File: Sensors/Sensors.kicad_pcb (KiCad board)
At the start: 4 copper layers, 17.6 x 37 mm, 11 parts, among them J1 Conn_01x05, J2 Conn_01x04, J3 Conn_01x02, U1 LIS2DE12, U2 MS5607-02BA

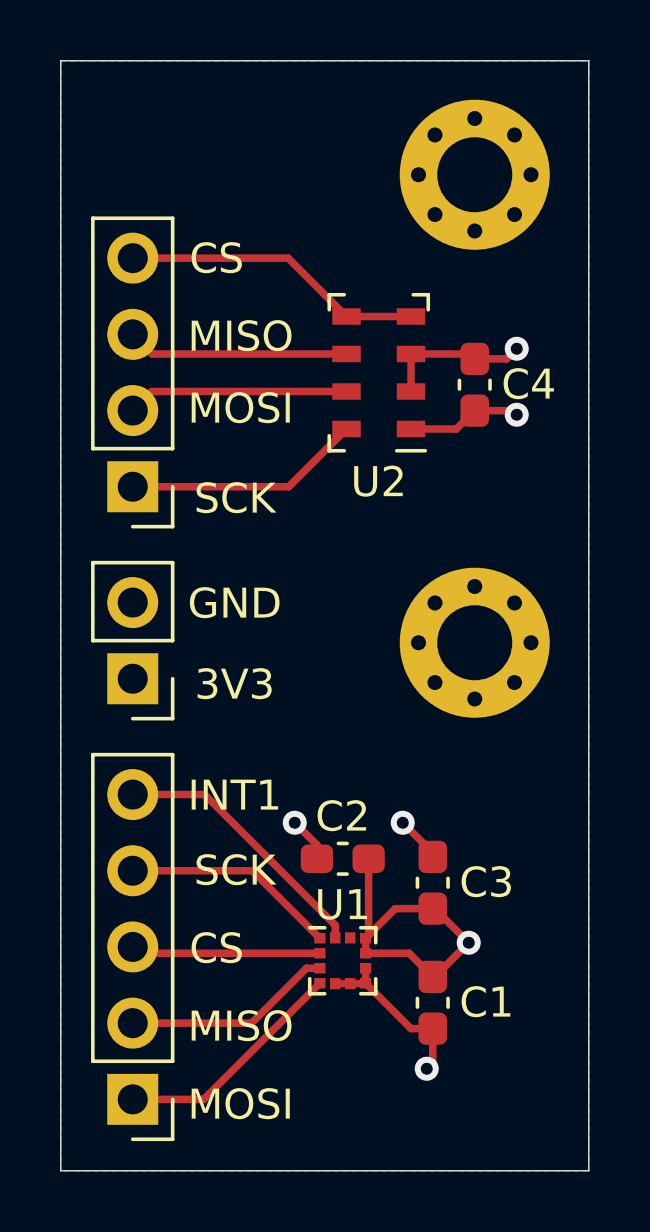
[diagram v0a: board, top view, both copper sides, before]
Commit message: Add files via upload
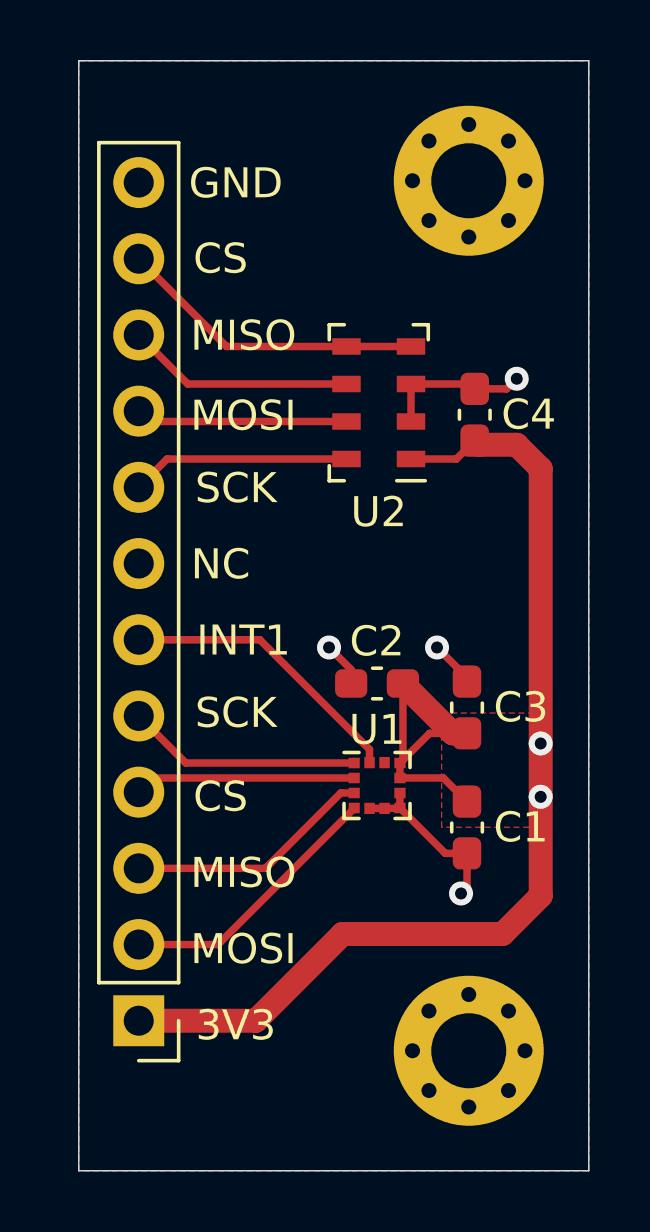
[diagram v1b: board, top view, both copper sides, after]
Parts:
- removed J2: Conn_01x04, Connector_PinHeader_2.54mm:PinHeader_1x04_P2.54mm_Vertical
- removed J3: Conn_01x02, Connector_PinHeader_2.54mm:PinHeader_1x02_P2.54mm_Vertical
- J1: value Conn_01x05 -> Conn_01x12; footprint Connector_PinHeader_2.54mm:PinHeader_1x05_P2.54mm_Vertical -> Connector_PinHeader_2.54mm:PinHeader_1x12_P2.54mm_Vertical
- moved H1 13.6 mm to (134.0, 106.0)
- moved C1 5.95 mm to (133.9, 98.6)
- moved C2 5.95 mm to (130.9, 93.8)
- moved C3 5.95 mm to (133.9, 94.6)
- moved U1 5.95 mm to (130.9, 97.2)
- moved J1 2.63 mm to (123.0, 105.0)
- moved C4 1.00 mm to (134.2, 84.8)
- moved U2 1.00 mm to (131.0, 84.4)
- moved H2 0.28 mm to (134.0, 77.0)
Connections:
- J1 pad 1: ACC_MOSI -> +3V3
- J1 pad 2: ACC_MISO -> ACC_MOSI
- J1 pad 3: ACC_CS -> ACC_MISO
- J1 pad 4: ACC_SCK -> ACC_CS
- J1 pad 5: INT1 -> ACC_SCK
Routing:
- net +3V3: track 15.6 -> 45.7 mm
- net ACC_MOSI: track 7.84 -> 9.07 mm
- net ACC_MISO: track 7.00 -> 8.22 mm
- net ACC_CS: track 6.32 -> 7.38 mm
- net INT1: track 8.98 -> 9.65 mm
- net ACC_SCK: track 7.17 -> 7.83 mm
- net BAR_SCK: track 7.92 -> 7.32 mm
- added copper zone on F.Cu, net +3V3
- added copper zone on B.Cu, net GND
- removed copper zone on B.Cu, net (none)
- removed copper zone on In2.Cu, net +3V3
- removed copper zone on In1.Cu, net GND
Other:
- board size 17.6 x 37 mm -> 17 x 37 mm
- copper layers 4 -> 2
- board text added: "NC"
